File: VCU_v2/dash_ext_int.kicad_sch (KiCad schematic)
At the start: 55 parts, among them Q3 SP8K80TB1, Q4 SP8K80TB1, Q5 SP8K80TB1

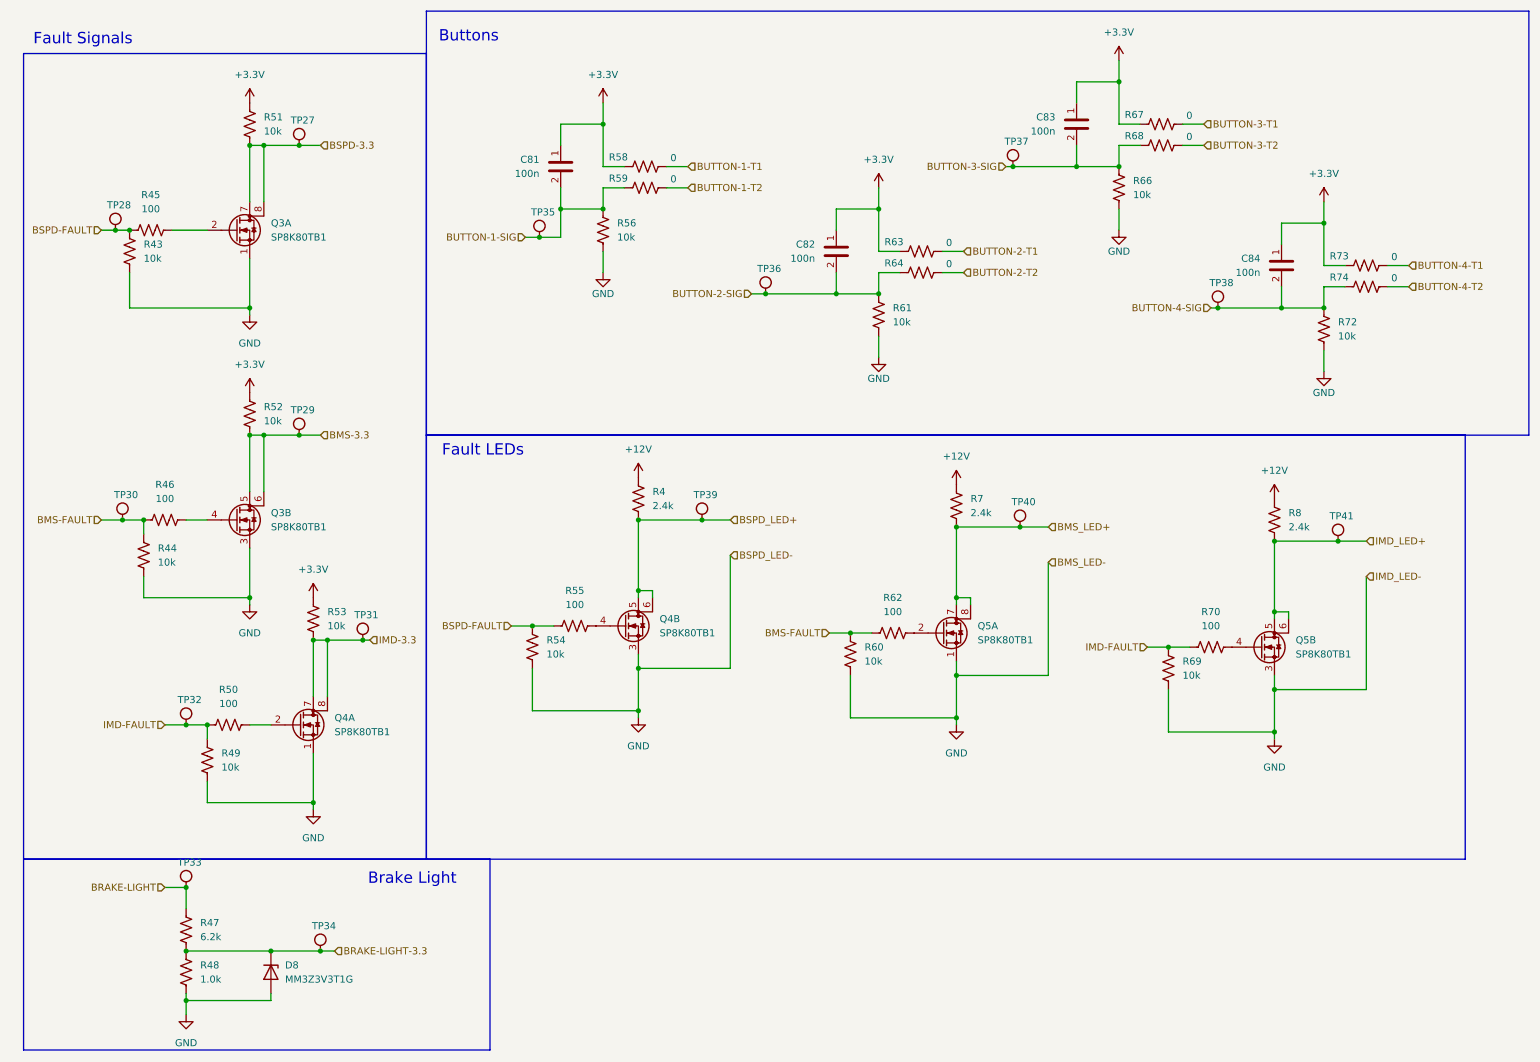
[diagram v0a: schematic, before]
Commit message: vcu v2 schematics done
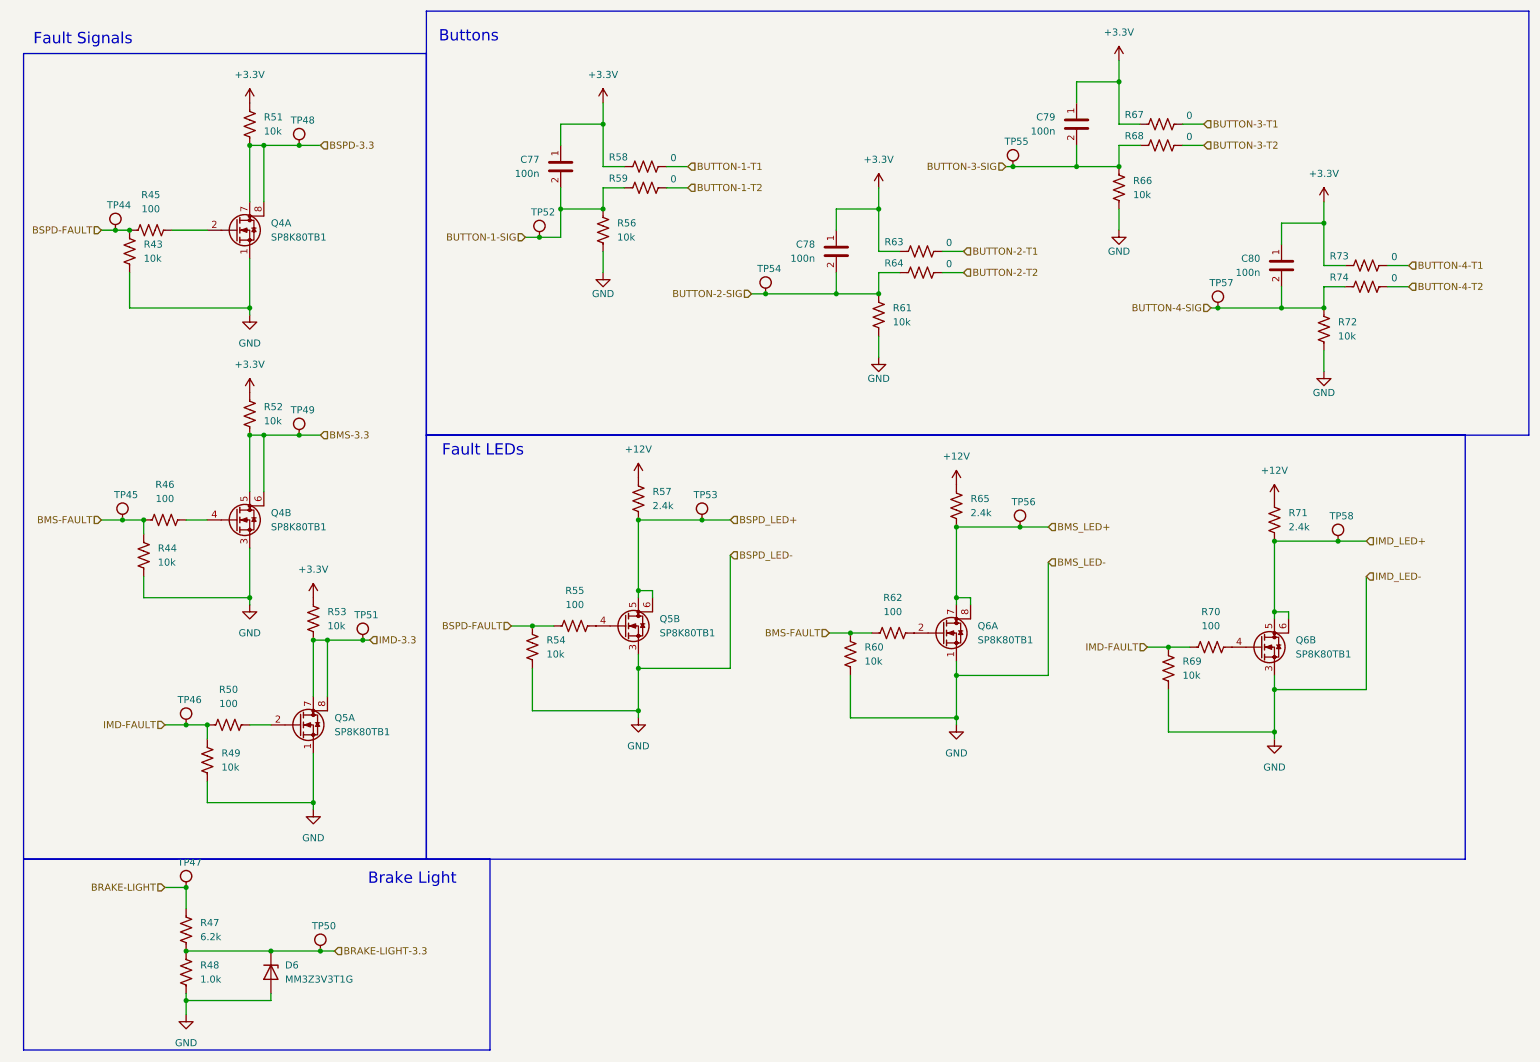
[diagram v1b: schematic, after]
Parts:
- renumbered C81 to C77, C82 to C78, C83 to C79, C84 to C80, D8 to D6, Q3 to Q4, Q4 to Q5, Q5 to Q6, R4 to R57, R7 to R65, R8 to R71, TP28 to TP44, TP30 to TP45, TP32 to TP46, TP33 to TP47, TP27 to TP48, TP29 to TP49, TP34 to TP50, TP31 to TP51, TP35 to TP52, TP39 to TP53, TP36 to TP54, TP37 to TP55, TP40 to TP56, TP38 to TP57, TP41 to TP58

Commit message: placements friggin 80% friggin done shoutout epstein
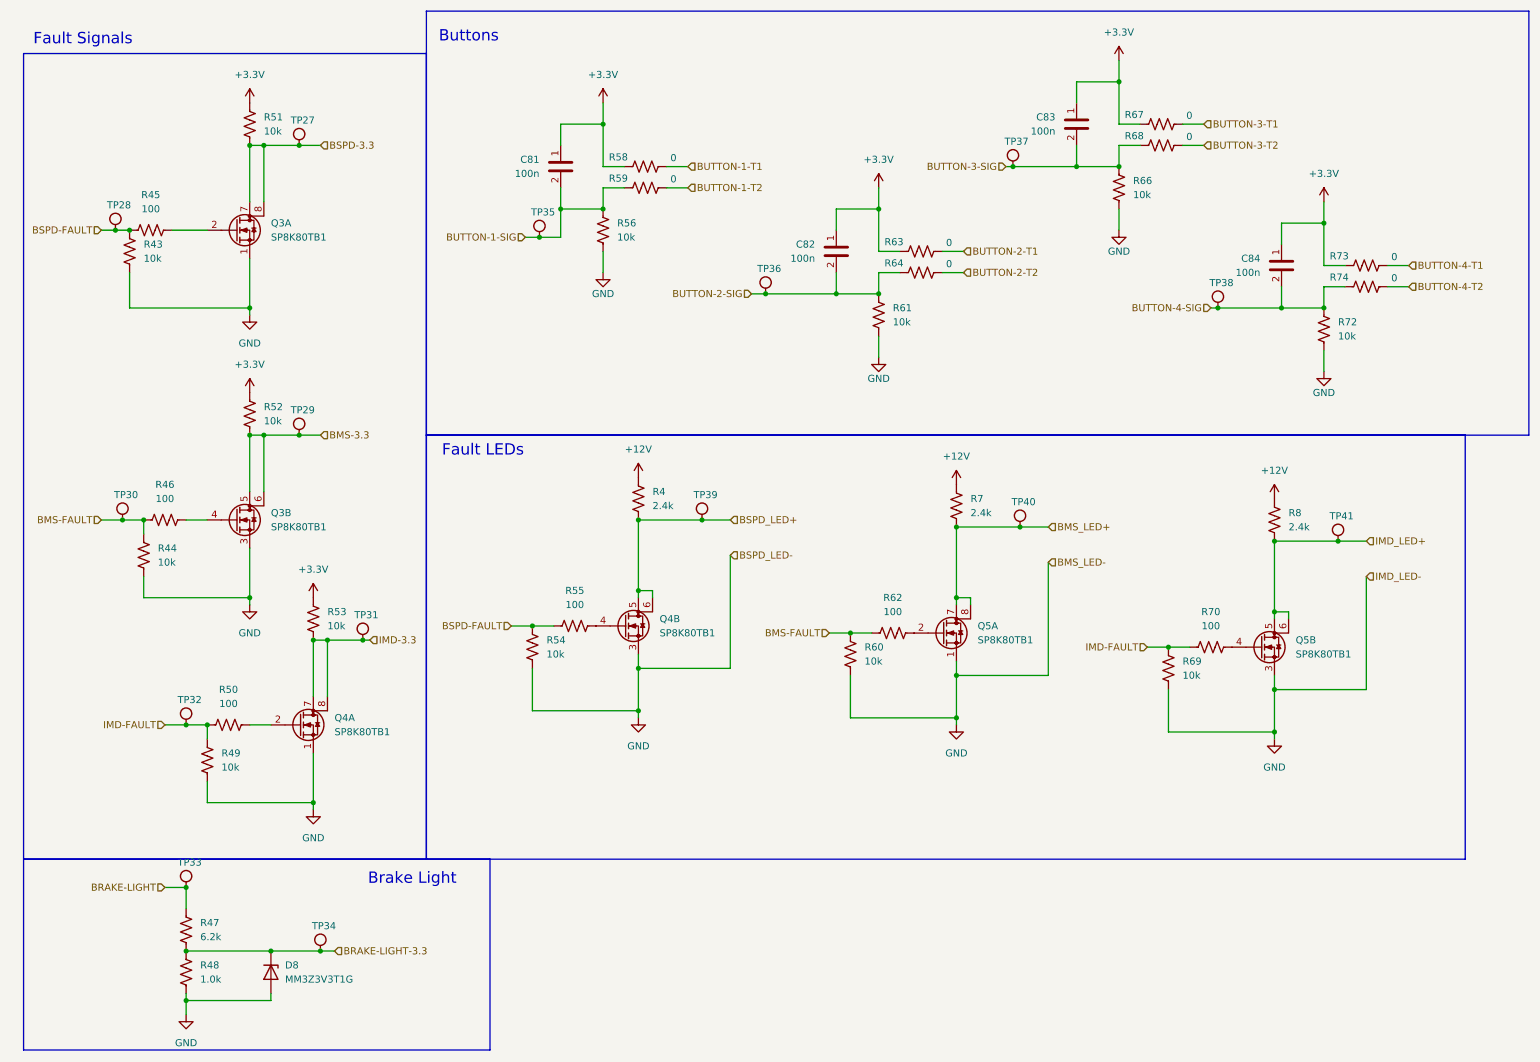
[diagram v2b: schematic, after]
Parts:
- renumbered C77 to C81, C78 to C82, C79 to C83, C80 to C84, D6 to D8, Q4 to Q3, Q5 to Q4, Q6 to Q5, R57 to R4, R65 to R7, R71 to R8, TP48 to TP27, TP44 to TP28, TP49 to TP29, TP45 to TP30, TP51 to TP31, TP46 to TP32, TP47 to TP33, TP50 to TP34, TP52 to TP35, TP54 to TP36, TP55 to TP37, TP57 to TP38, TP53 to TP39, TP56 to TP40, TP58 to TP41
